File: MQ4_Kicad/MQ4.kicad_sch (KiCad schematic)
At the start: 11 parts, among them J1 Motor_2, J2 Motor_4, J3 Motor_1, J4 Motor_3, J6 Battery_input, J8 Conn_01x03, U5 LD1117S33TR_SOT223

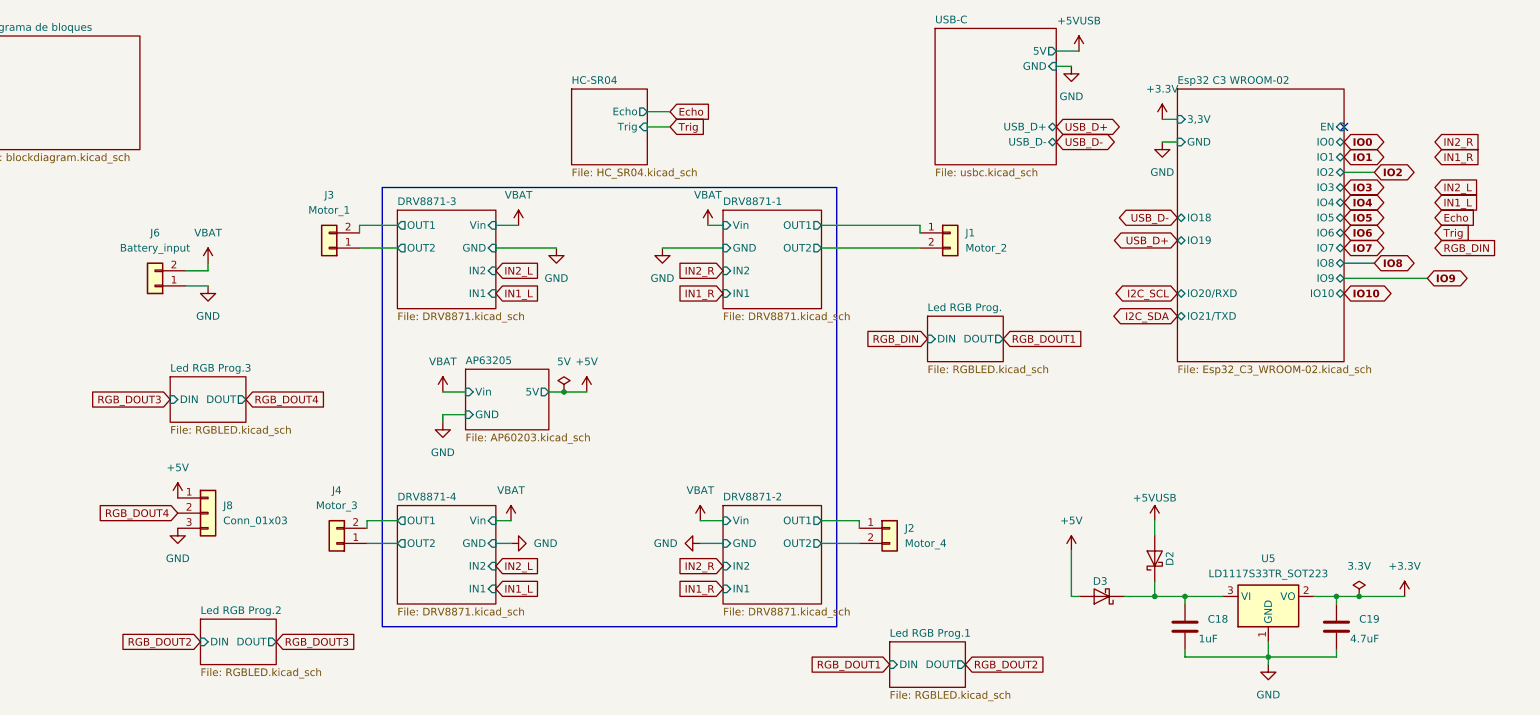
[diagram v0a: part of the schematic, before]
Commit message: Ajustes 3
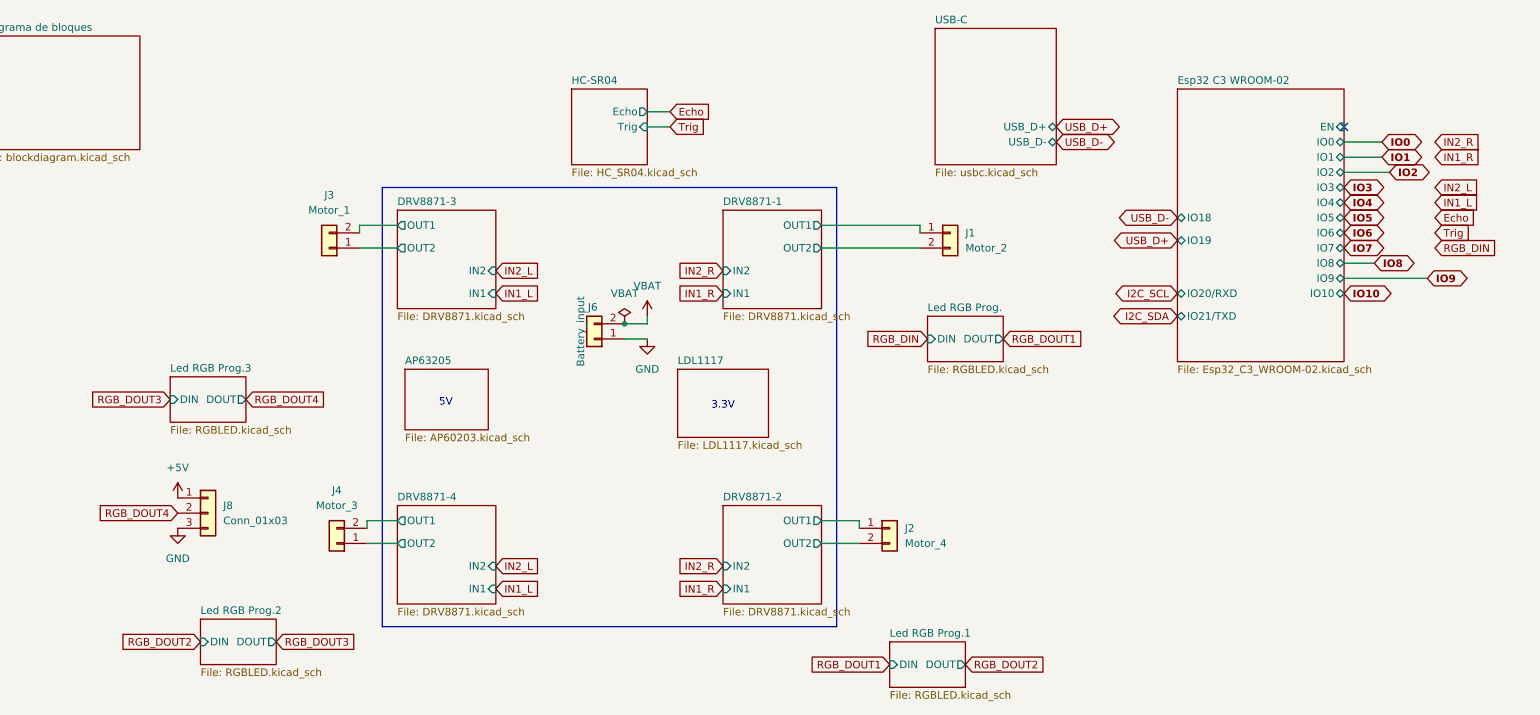
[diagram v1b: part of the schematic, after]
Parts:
- removed C18: 1uF, Capacitor_SMD:C_0805_2012Metric, symbol Device:C
- removed C19: 4.7uF, Capacitor_SMD:C_0805_2012Metric, symbol Device:C
- removed D2, D3: SMD22PL, Diode_SMD:D_SOD-123F, symbol Diode:PMEG6010CEH
- removed U5: LD1117S33TR_SOT223, Package_TO_SOT_SMD:SOT-223-3_TabPin2, symbol Regulator_Linear:LD1117S33TR_SOT223
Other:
- added sheet LDL1117 (LDL1117.kicad_sch)
- sheet AP63205 ports: added none; removed 5V, GND, Vin
- sheet DRV8871-1 ports: added none; removed GND, Vin
- sheet DRV8871-2 ports: added none; removed GND, Vin
- sheet DRV8871-3 ports: added none; removed GND, Vin
- sheet DRV8871-4 ports: added none; removed GND, Vin
- sheet Esp32 C3 WROOM-02 ports: added none; removed 3,3V, GND
- sheet USB-C ports: added none; removed 5V, GND
- note added: "3.3V"
- note added: "5V"
- moved on the sheet: J6
